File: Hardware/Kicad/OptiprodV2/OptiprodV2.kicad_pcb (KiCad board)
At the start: 2 copper layers, 27 parts, among them U1 MCP6002-xMC, U2 BME280, U3 TL082, U4 TL082

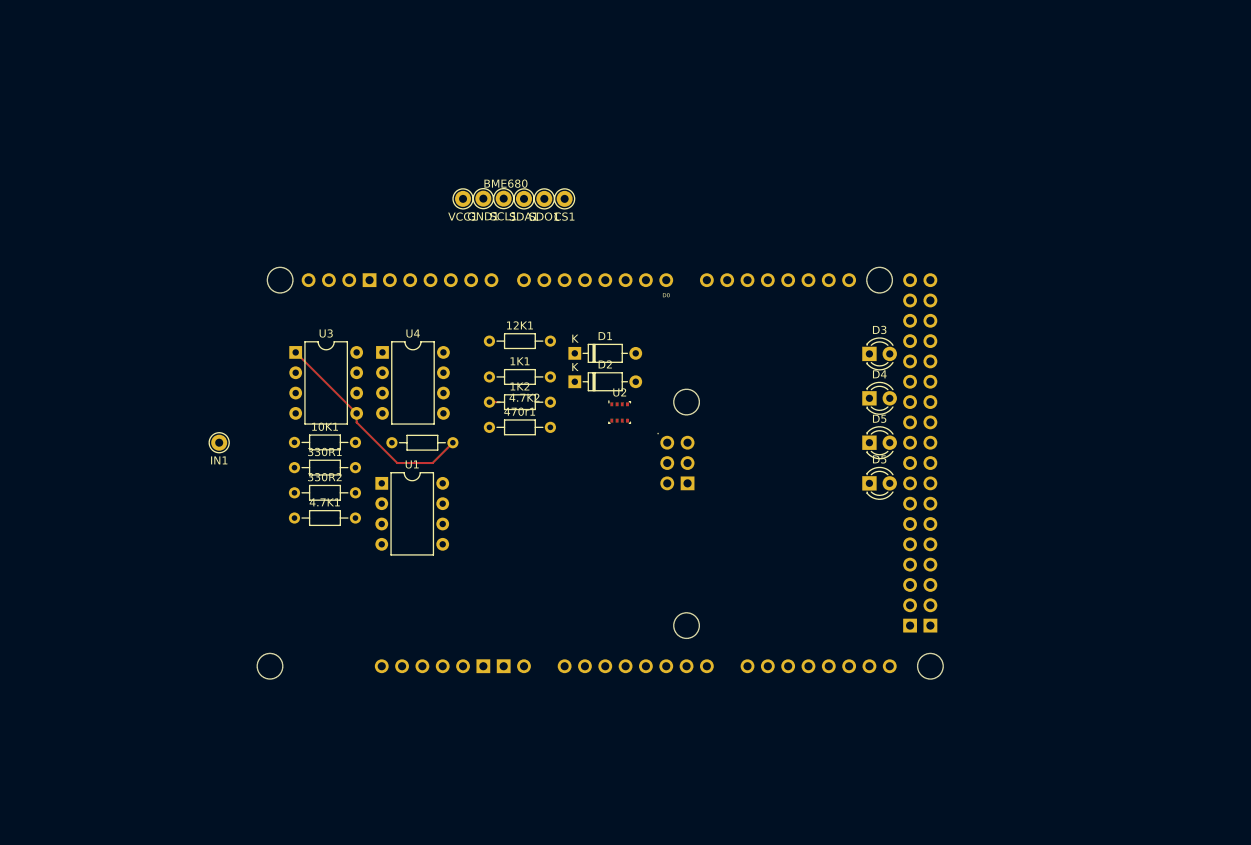
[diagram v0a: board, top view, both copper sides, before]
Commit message: modifiedkicad
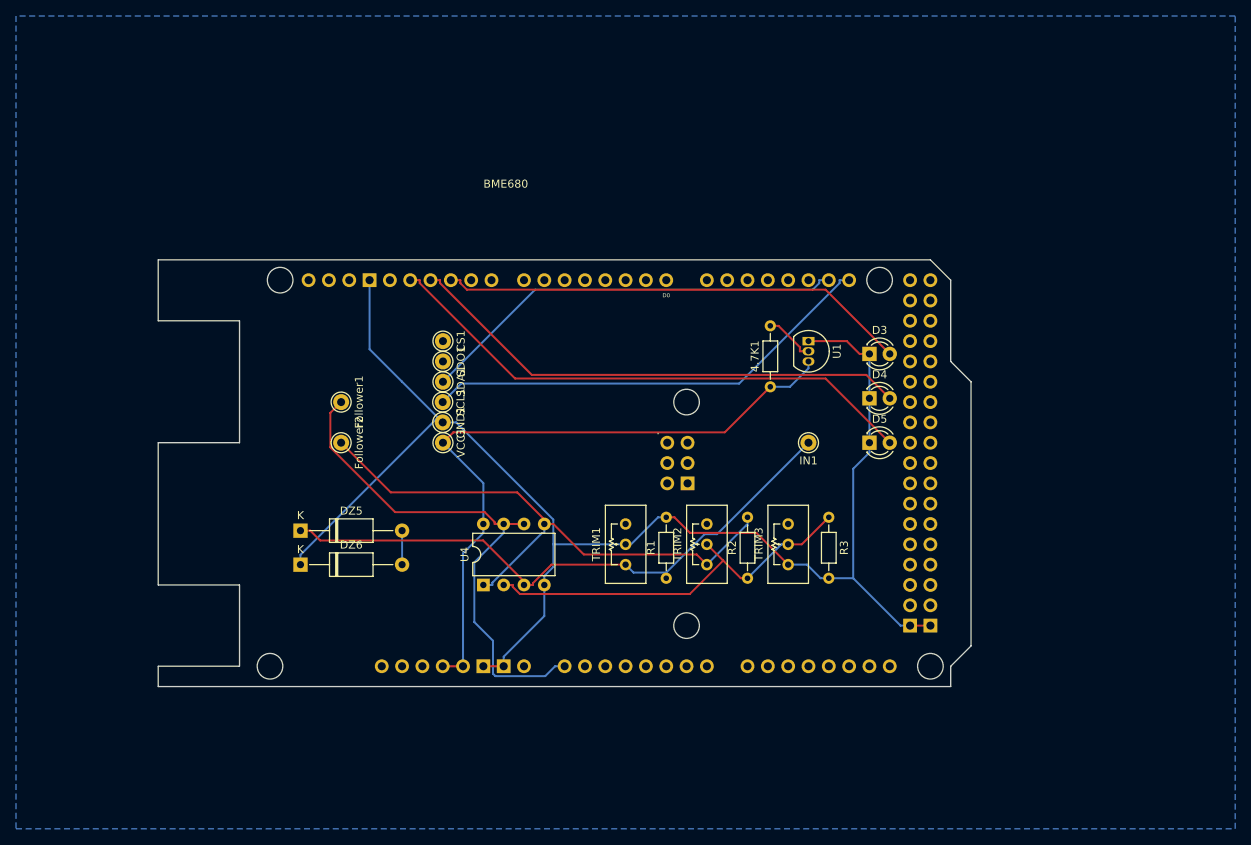
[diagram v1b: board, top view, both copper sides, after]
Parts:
- removed 10K1, 12K1, 1K1, 1K2, 330R1, 330R2, 4.7K2, 470r1: R, Resistor_THT:R_Axial_DIN0204_L3.6mm_D1.6mm_P7.62mm_Horizontal
- removed D1, D2: D_Zener, Diode_THT:D_DO-35_SOD27_P7.62mm_Horizontal
- removed the D5 at (182.9, 83.8)
- removed U2: BME280, Package_LGA:Bosch_LGA-8_2.5x2.5mm_P0.65mm_ClockwisePinNumbering
- removed U3: TL082, Package_DIP:DIP-8_W7.62mm
- added DZ5: 1N4733, Diode_THT:D_A-405_P12.70mm_Horizontal, F.Cu at (111.8, 89.7)
- added DZ6: 1N4733, Diode_THT:D_A-405_P12.70mm_Horizontal, F.Cu at (111.8, 94.0)
- added Follower1: MountingHole_Pad, Connector_Pin:Pin_D1.0mm_L10.0mm, F.Cu at (116.8, 73.7)
- added Follower2: MountingHole_Pad, Connector_Pin:Pin_D1.0mm_L10.0mm, F.Cu at (116.8, 78.7)
- added R1: R, Resistor_THT:R_Axial_DIN0204_L3.6mm_D1.6mm_P7.62mm_Horizontal, F.Cu at (157.5, 95.7)
- added R2: R, Resistor_THT:R_Axial_DIN0204_L3.6mm_D1.6mm_P7.62mm_Horizontal, F.Cu at (167.6, 95.7)
- added R3: R, Resistor_THT:R_Axial_DIN0204_L3.6mm_D1.6mm_P7.62mm_Horizontal, F.Cu at (177.8, 88.1)
- added TRIM1: TrimPot_T73YEt_1k, PCM_Potentiometer_THT_US_AKL:Potentiometer_Bourns_3296W_Vertical, F.Cu at (152.4, 88.9)
- added TRIM2: TrimPot_T73YEt_1k, PCM_Potentiometer_THT_US_AKL:Potentiometer_Bourns_3296W_Vertical, F.Cu at (162.6, 88.9)
- added TRIM3: TrimPot_T73YEt_1k, PCM_Potentiometer_THT_US_AKL:Potentiometer_Bourns_3296W_Vertical, F.Cu at (172.7, 88.9)
- U1: value MCP6002-xMC -> DS18B20; footprint Package_DIP:DIP-8_W7.62mm -> Package_TO_SOT_THT:TO-92_Inline
- moved IN1 73.7 mm to (175.3, 78.7)
- moved 4.7K1 61.7 mm to (170.5, 71.8), turned to 90 degrees
- moved U1 56.2 mm to (175.3, 66.0), turned to -90 degrees
- moved U4 31.7 mm to (134.6, 96.5), turned to 90 degrees
- moved VCC1 30.6 mm to (129.6, 78.7), turned to 90 degrees
- moved GND1 28.4 mm to (129.5, 76.2), turned to 90 degrees
- moved SCL1 26.5 mm to (129.5, 73.7), turned to 90 degrees
- moved SDA1 25.0 mm to (129.6, 71.1), turned to 90 degrees
- moved SDO1 23.9 mm to (129.6, 68.6), turned to 90 degrees
- moved CS1 23.4 mm to (129.6, 66.0), turned to 90 degrees
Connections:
- 4.7K1 pad 1: Net-(U4A--) -> VCC
- 4.7K1 pad 2: Net-(U4B-+) -> Net-(U1-DQ)
- A2 pad 5V1: Net-(U1C-V+) -> VCC
- A2 pad A1: Net-(470r1-Pad2) -> unconnected-(A2-PadA1)
- A2 pad D20: unconnected-(A2-D20/SDA-PadD20) -> Net-(A2-D20/SDA)
- A2 pad D21: unconnected-(A2-D21/SCL-PadD21) -> Net-(A2-D21/SCL)
- SCL1 pad 1: unconnected-(SCL1-Pad1) -> Net-(A2-D21/SCL)
- SDA1 pad 1: unconnected-(SDA1-Pad1) -> Net-(A2-D20/SDA)
- U1 pad 1: Net-(470r1-Pad2) -> GND
- U1 pad 2: Net-(U1A--) -> Net-(U1-DQ)
- U1 pad 3: Net-(DZ3-K) -> VCC
- U4 pad 1: Net-(U4B-+) -> Net-(TRIM2-Right)
- U4 pad 2: Net-(U4A--) -> Net-(TRIM2-Center)
- U4 pad 5: Net-(U4B-+) -> Net-(TRIM2-Right)
- U4 pad 8: Net-(U1C-V+) -> VCC
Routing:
- net GND: track 0.00 -> 180.7 mm
- net VCC: track 0.00 -> 84.0 mm
- net Net-(DZ5-K): track 0.00 -> 75.8 mm
- net Net-(TRIM2-Right): track 0.00 -> 72.3 mm
- net Net-(D5-A): track 0.00 -> 68.6 mm
- net Net-(U4B--): track 0.00 -> 65.3 mm
- net Net-(D4-A): track 0.00 -> 63.7 mm
- net Net-(D3-A): track 0.00 -> 58.9 mm
- net Net-(A2-D21/SCL): track 0.00 -> 57.3 mm
- net Net-(A2-D20/SDA): track 0.00 -> 53.7 mm
- net Net-(TRIM2-Center): track 0.00 -> 49.9 mm
- net Net-(U3B-+): track 27.1 -> 0.00 mm
- net Net-(U1-DQ): track 0.00 -> 6.39 mm
- net Net-(DZ5-A): track 0.00 -> 4.25 mm
- net Net-(12K1-Pad2): track 1.32 -> 0.00 mm
- added copper zone on B.Cu, net GND
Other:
- board outline added: 101.6 x 53.3 mm
